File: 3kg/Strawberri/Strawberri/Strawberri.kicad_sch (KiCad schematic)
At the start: 68 parts, among them J1 Screw_Terminal_01x08, J13 Screw_Terminal_01x03, J14 Screw_Terminal_01x03, J15 Conn_02x05_Odd_Even, J16 Screw_Terminal_01x03, J17 Screw_Terminal_01x03, J18 Screw_Terminal_01x03, J19 Screw_Terminal_01x03, J2 Screw_Terminal_01x03, J20 Screw_Terminal_01x03, J21 Screw_Terminal_01x03, J3 Screw_Terminal_01x03, J4 Screw_Terminal_01x03, J5 Screw_Terminal_01x03, J6 Screw_Terminal_01x03, J7 Battery, J8 Screw_Terminal_01x03, SW1 SW_SPDT, SW2 SW_DIP_x03, U1 DEV-16771, U10 SFH617A-3, U2 SFH617A-3, U3 SFH617A-3, U4 SFH617A-3, U5 SFH617A-3, U6 SFH617A-3, U7 SFH617A-3, U9 R-78K5.0-0.5 (vr 5v)

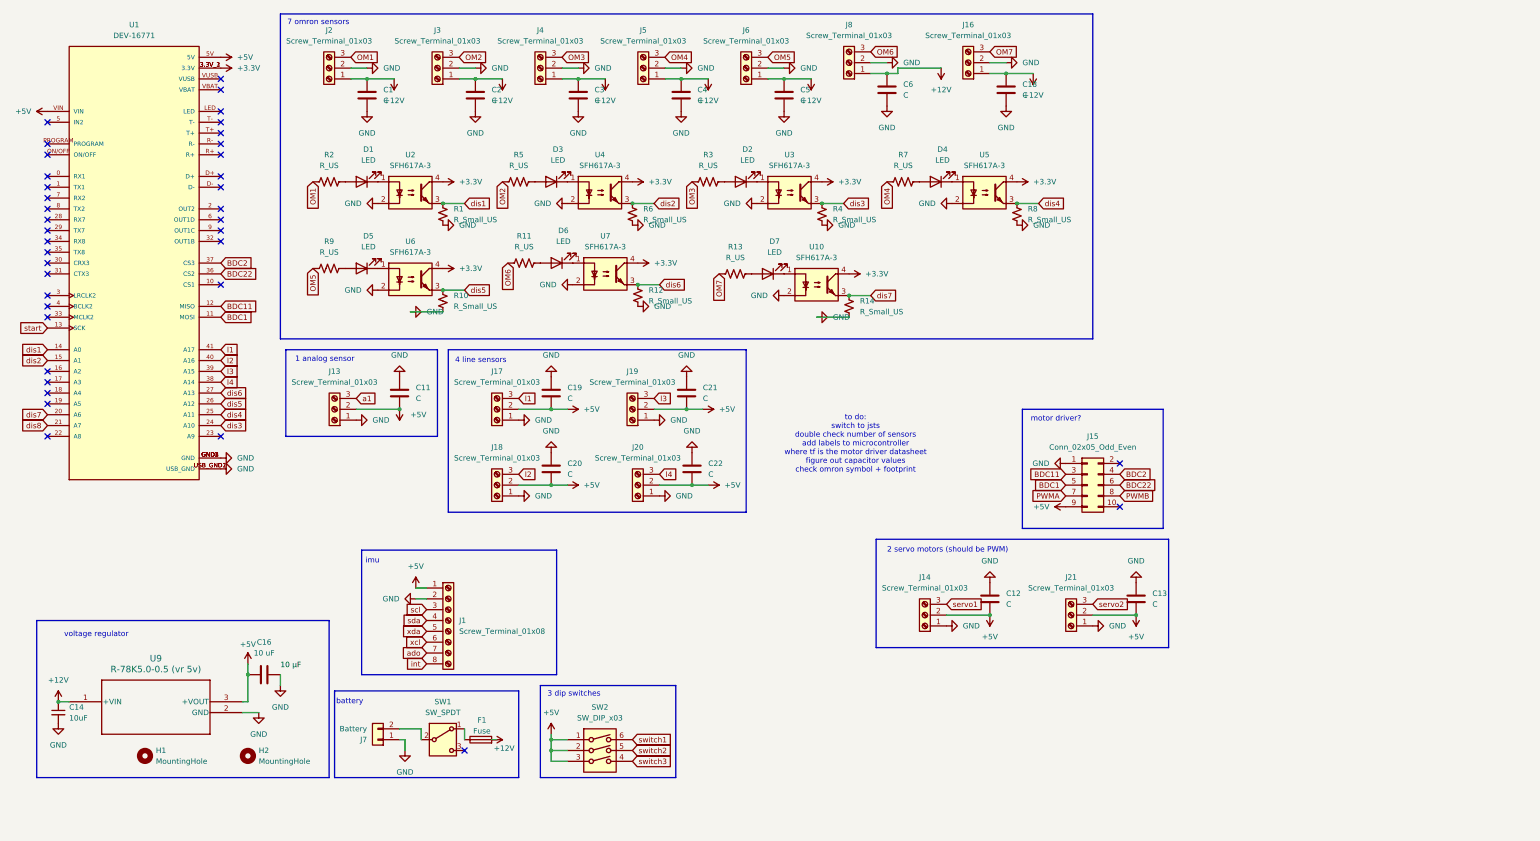
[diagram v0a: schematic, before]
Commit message: did some todos
yeah
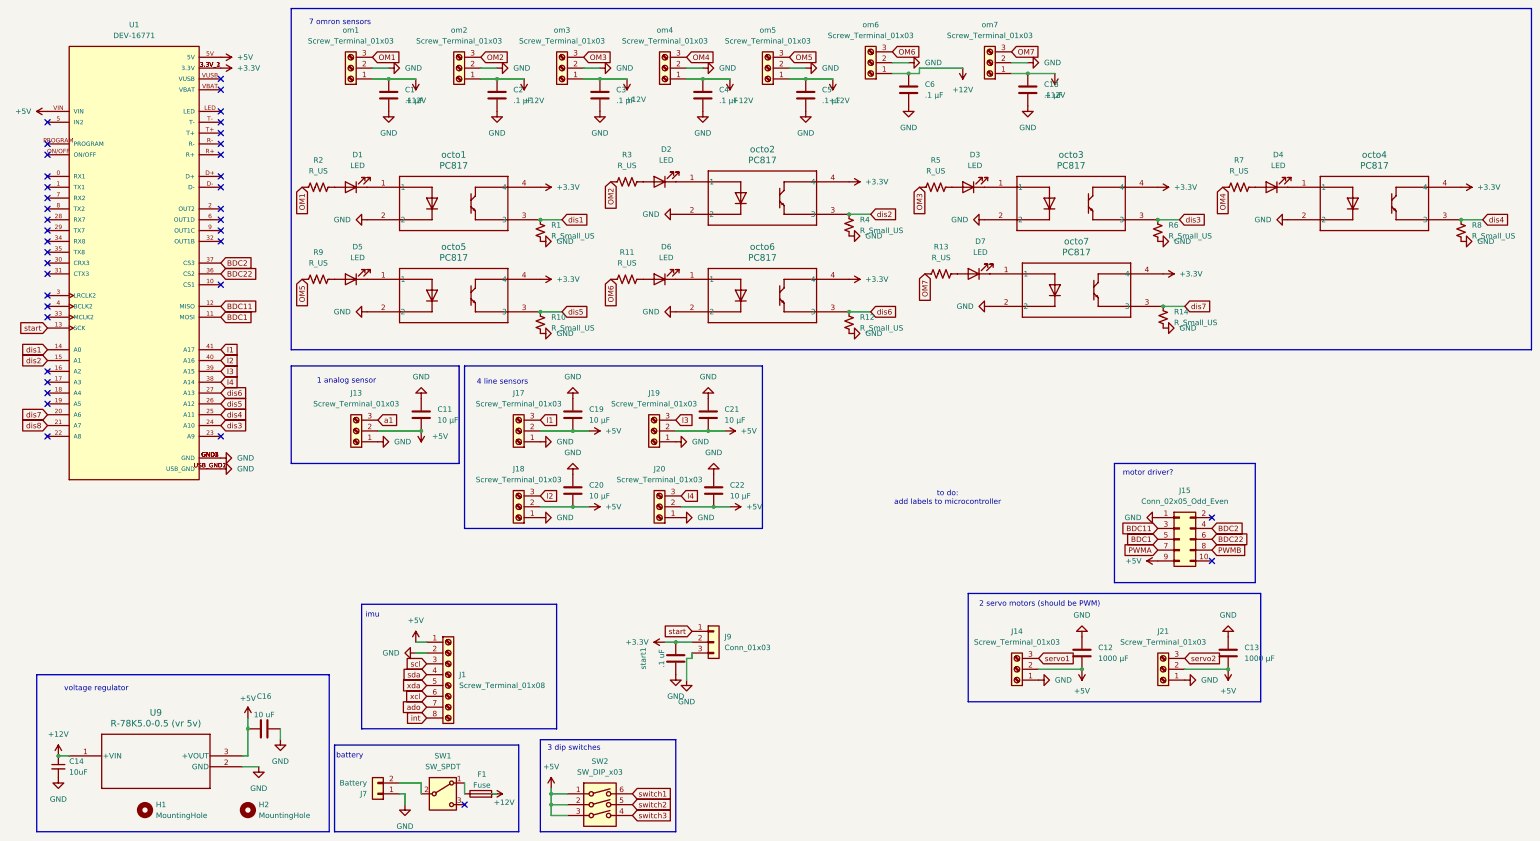
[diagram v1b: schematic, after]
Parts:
- removed U10, U2, U3, U4, U5, U6, U7: SFH617A-3, Package_DIP:DIP-4_W7.62mm, symbol Isolator:SFH617A-3
- added J9: Conn_01x03, TerminalBlock:TerminalBlock_Xinya_XY308-2.54-3P_1x03_P2.54mm_Horizontal, symbol Connector_Generic:Conn_01x03
- added octo1, octo2, octo3, octo4, octo5, octo6, octo7: PC817, Connector_Molex:Molex_Pico-EZmate_Slim_202656-0021_1x02-1MP_P1.20mm_Vertical, symbol 2026-01-23_00-22-03:PC817
- added start1: .1 uF, Capacitor_SMD:C_0805_2012Metric, symbol Device:C
- C1, C18, C2, C3, C4, C5, C6: value C -> .1 µF
- C11, C19, C20, C21, C22: value C -> 10 µF
- C12, C13: value C -> 1000 µF
- J1: footprint (none) -> Connector_JST:JST_PH_B8B-PH-K_1x08_P2.00mm_Vertical
- J13, J17, J18, J19, J20: footprint TerminalBlock:TerminalBlock_Xinya_XY308-2.54-3P_1x03_P2.54mm_Horizontal -> Connector_JST:JST_PH_B3B-PH-K_1x03_P2.00mm_Vertical
- J7: footprint Connector_AMASS:AMASS_XT30U-F_1x02_P5.0mm_Vertical -> Connector_JST:JST_PH_B3B-PH-K_1x03_P2.00mm_Vertical
- R10, R12, R14, R4, R6, R8: footprint Resistor_SMD:R_0805_2012Metric -> Resistor_SMD:R_0805_2012Metric_Pad1.20x1.40mm_HandSolder
- SW2: footprint (none) -> switch:SW_219-3LPSTR
- om1: renamed from J2; footprint TerminalBlock:TerminalBlock_Xinya_XY308-2.54-3P_1x03_P2.54mm_Horizontal -> Connector_JST:JST_PH_B3B-PH-K_1x03_P2.00mm_Vertical
- om2: renamed from J3; footprint TerminalBlock:TerminalBlock_Xinya_XY308-2.54-3P_1x03_P2.54mm_Horizontal -> Connector_JST:JST_PH_B3B-PH-K_1x03_P2.00mm_Vertical
- om3: renamed from J4; footprint TerminalBlock:TerminalBlock_Xinya_XY308-2.54-3P_1x03_P2.54mm_Horizontal -> Connector_JST:JST_PH_B3B-PH-K_1x03_P2.00mm_Vertical
- om4: renamed from J5; footprint TerminalBlock:TerminalBlock_Xinya_XY308-2.54-3P_1x03_P2.54mm_Horizontal -> Connector_JST:JST_PH_B3B-PH-K_1x03_P2.00mm_Vertical
- om5: renamed from J6; footprint TerminalBlock:TerminalBlock_Xinya_XY308-2.54-3P_1x03_P2.54mm_Horizontal -> Connector_JST:JST_PH_B3B-PH-K_1x03_P2.00mm_Vertical
- om6: renamed from J8; footprint TerminalBlock:TerminalBlock_Xinya_XY308-2.54-3P_1x03_P2.54mm_Horizontal -> Connector_JST:JST_PH_B3B-PH-K_1x03_P2.00mm_Vertical
- om7: renamed from J16; footprint TerminalBlock:TerminalBlock_Xinya_XY308-2.54-3P_1x03_P2.54mm_Horizontal -> Connector_JST:JST_PH_B3B-PH-K_1x03_P2.00mm_Vertical
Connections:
- net +3.3V: now also J9.2 (Pin_2), octo1.4, octo2.4, octo3.4, octo4.4, octo5.4, octo6.4, octo7.4, start1.2
- net GND: now also J9.3 (Pin_3), octo1.2, octo2.2, octo3.2, octo4.2, octo5.2, octo6.2, octo7.2, start1.1
- net OM2: now also R3.1; no longer R5.1
- net OM3: now also R5.1; no longer R3.1
- net dis1: now also octo1.3
- net dis2: now also R4.1, octo2.3; no longer R6.1
- net dis3: now also R6.1, octo3.3; no longer R4.1
- net dis4: now also octo4.3
- net dis5: now also octo5.3
- net dis6: now also octo6.3
- net dis7: now also octo7.3
- net start: now also J9.1 (Pin_1)
- net at D4.1 (K): now also octo4.1
- net at D6.1 (K): now also octo6.1
- net at D7.1 (K): now also octo7.1
- net at D5.1 (K): now also octo5.1
- net at D2.1 (K): now also octo2.1
- net at D3.1 (K): now also octo3.1
- net at D1.1 (K): now also octo1.1
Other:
- note added: "to do: add labels to microcontroller"
- note removed: "to do: switch to jsts double check number of sensors add labels to microcontroller where tf is the motor driver datasheet figure out capacitor values check omron symbol + footprint"
- moved on the sheet: C1, C11, C12, C13, C14, C16, C18, C19, C2, C20, C21, C22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
